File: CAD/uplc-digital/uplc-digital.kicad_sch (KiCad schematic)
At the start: 34 parts, among them J1 Conn_01x06_Pin, J2 SM12B-GHS-TB(LF)(SN), U1 AP63201WU, U2 TBD62003AFWG, U3 ESP32-C3-WROOM-02, Y1 32.768khz 3215 12.5pf

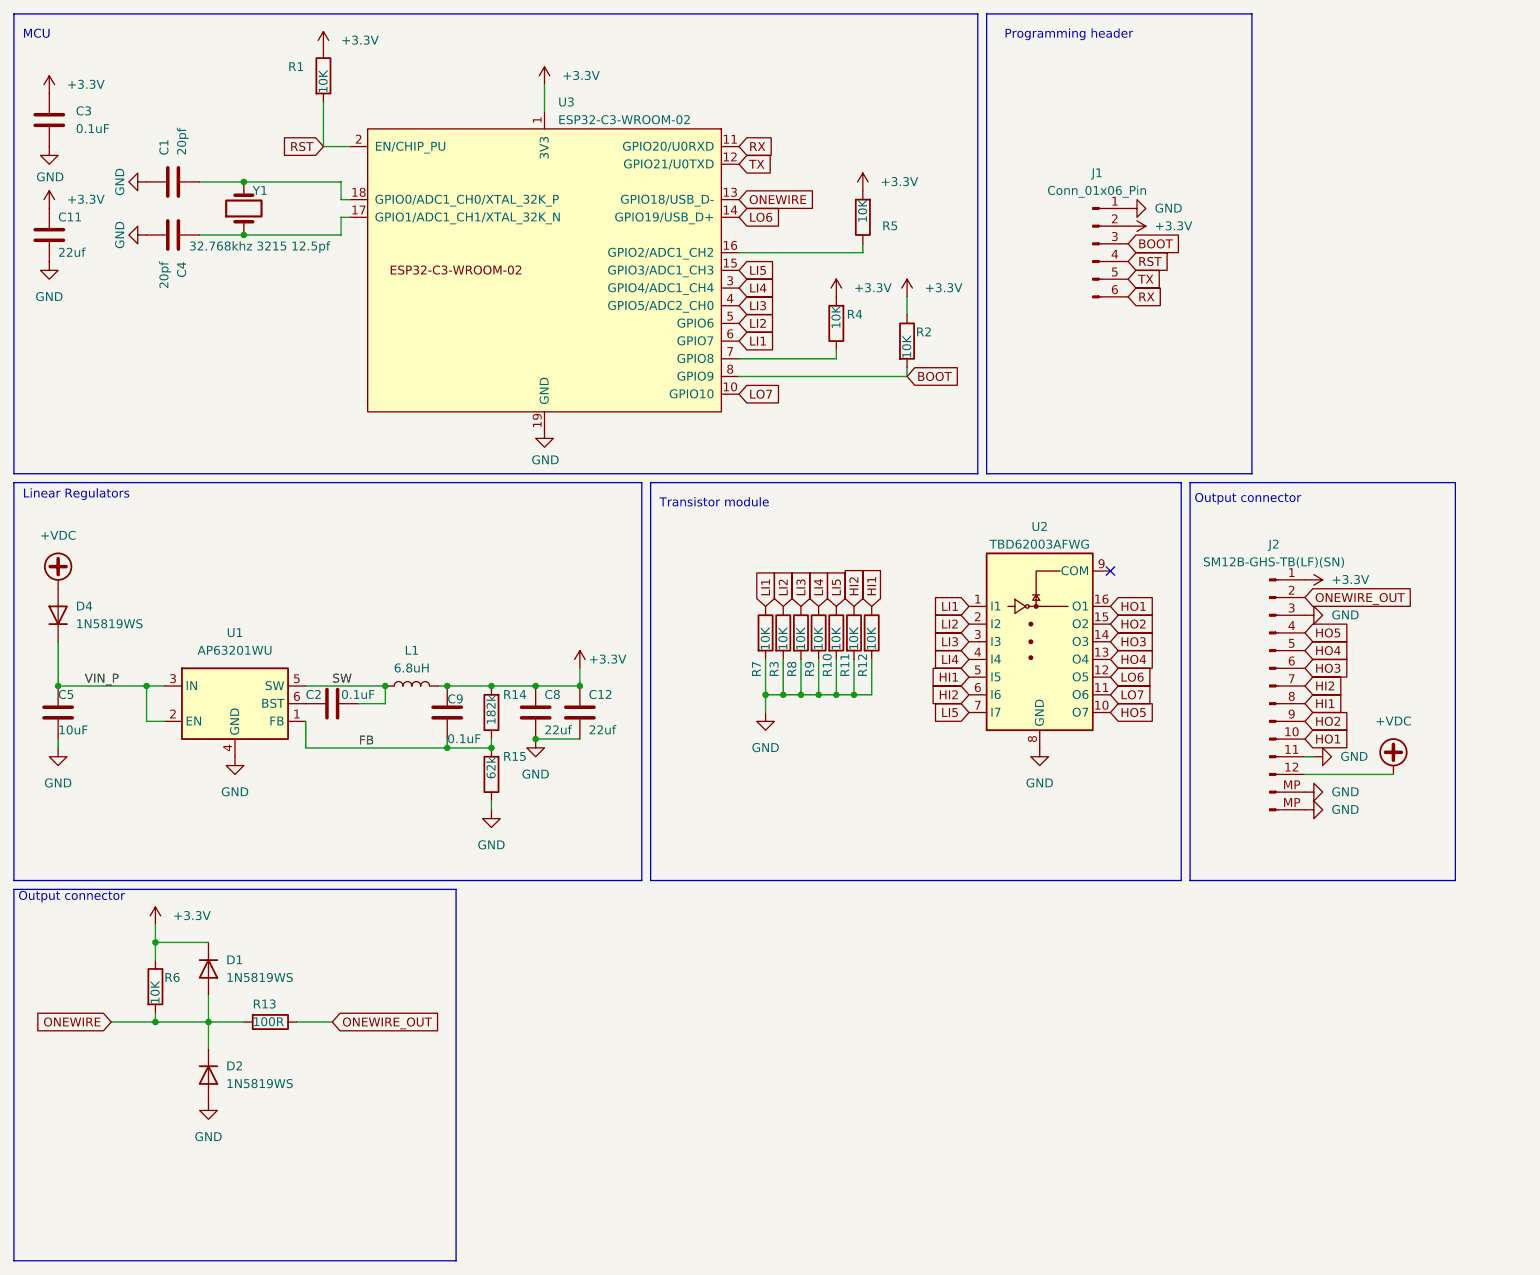
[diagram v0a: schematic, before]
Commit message: WIP rev 1.1
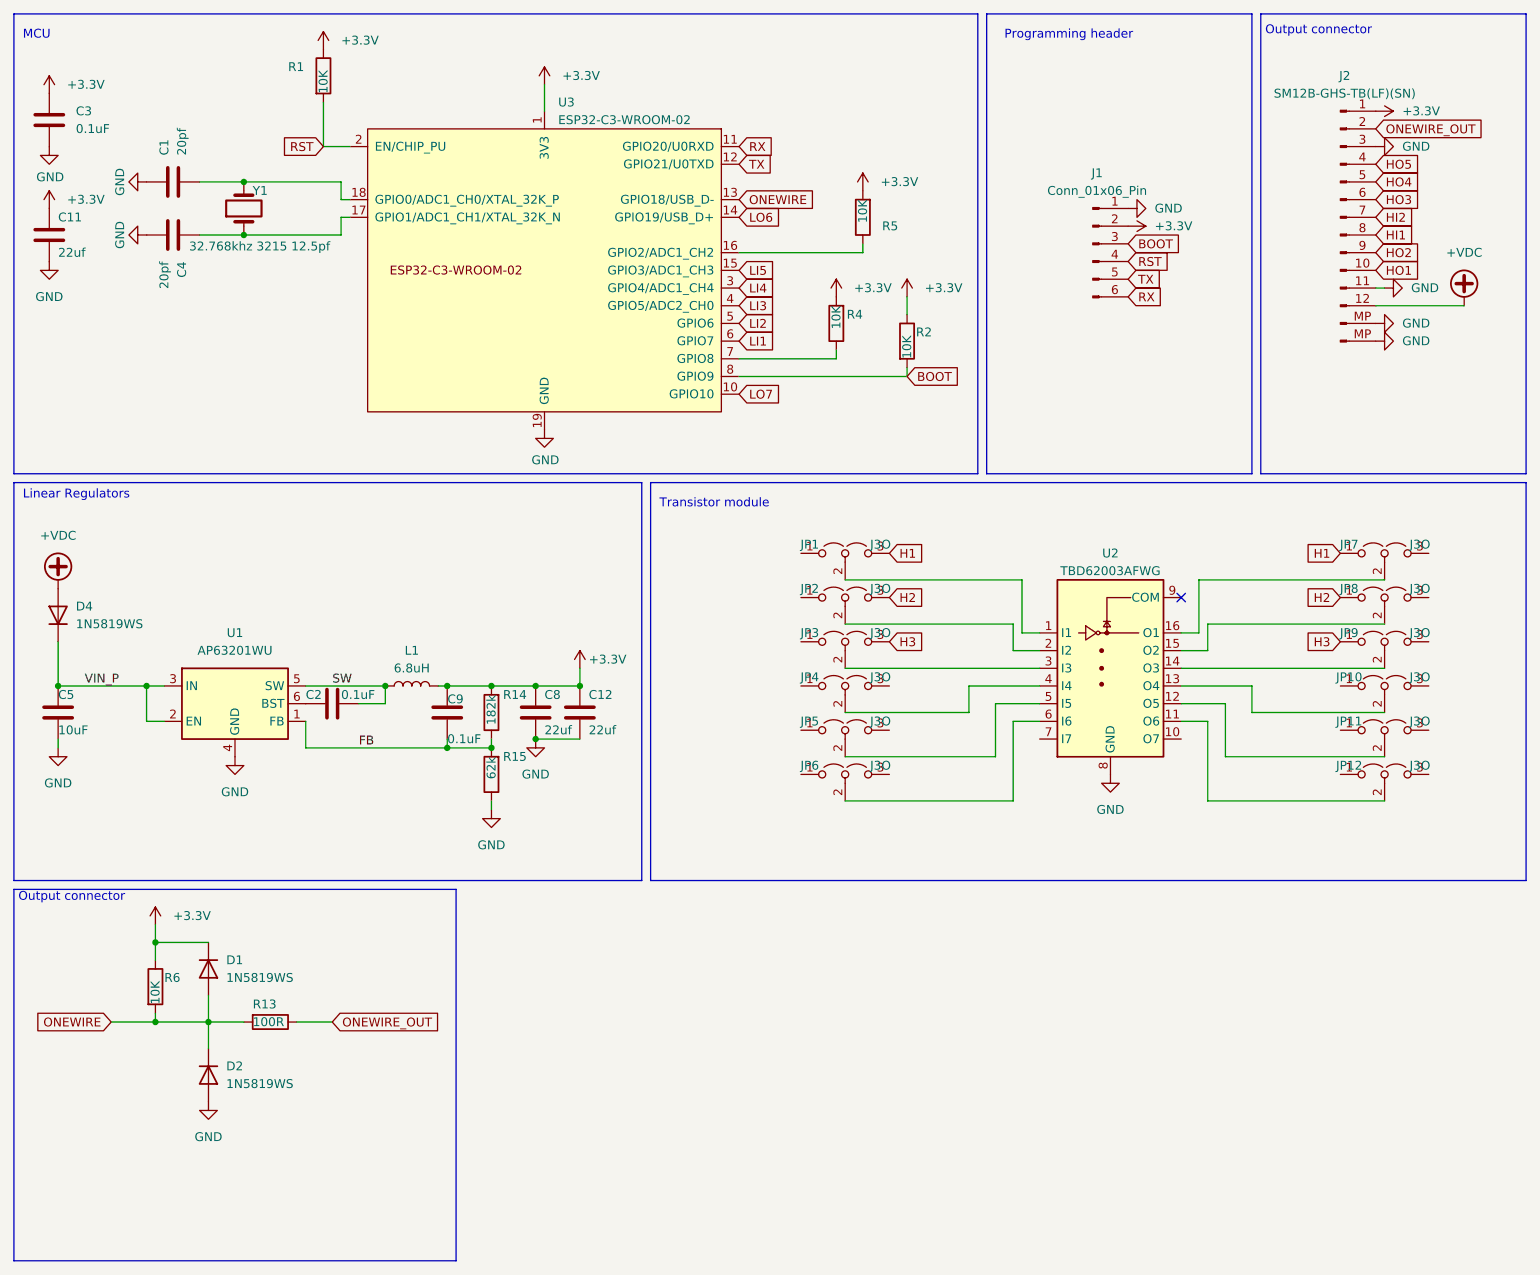
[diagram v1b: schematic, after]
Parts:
- removed R10, R11, R12, R3, R7, R8, R9: 10K, Resistor_SMD:R_0402_1005Metric, symbol Library:R
- added JP1, JP10, JP11, JP12, JP2, JP3, JP4, JP5, JP6, JP7, JP8, JP9: J3O, Jumper:SolderJumper-3_P1.3mm_Open_Pad1.0x1.5mm_NumberLabels, symbol Jumper:Jumper_3_Open
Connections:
- net HI1: no longer U2.5 (I5)
- net HI2: no longer U2.6 (I6)
- net HO1: no longer U2.16 (O1)
- net HO2: no longer U2.15 (O2)
- net HO3: no longer U2.14 (O3)
- net HO4: no longer U2.13 (O4)
- net HO5: no longer U2.10 (O7)
- net LI1: no longer U2.1 (I1)
- net LI2: no longer U2.2 (I2)
- net LI3: no longer U2.3 (I3)
- net LI4: no longer U2.4 (I4)
- net LI5: no longer U2.7 (I7)
- net LO6: no longer U2.12 (O5)
- net LO7: no longer U2.11 (O6)
- new net: JP10.2 (C), U2.13 (O4)
- new net: JP6.2 (C), U2.6 (I6)
- new net: JP3.2 (C), U2.3 (I3)
- new net: JP1.2 (C), U2.1 (I1)
- new net: JP7.2 (C), U2.16 (O1)
- new net: JP11.2 (C), U2.12 (O5)
- new net: JP4.2 (C), U2.4 (I4)
- new net: JP5.2 (C), U2.5 (I5)
- new net: JP8.2 (C), U2.15 (O2)
- new net: JP2.2 (C), U2.2 (I2)
- new net: JP9.2 (C), U2.14 (O3)
- new net: JP12.2 (C), U2.11 (O6)
- new net H1: JP1.3 (B), JP7.1 (A)
- new net H2: JP2.3 (B), JP8.1 (A)
- new net H3: JP3.3 (B), JP9.1 (A)
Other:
- moved on the sheet: J2, U2

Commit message: Rev 1.1 Schem PCB done
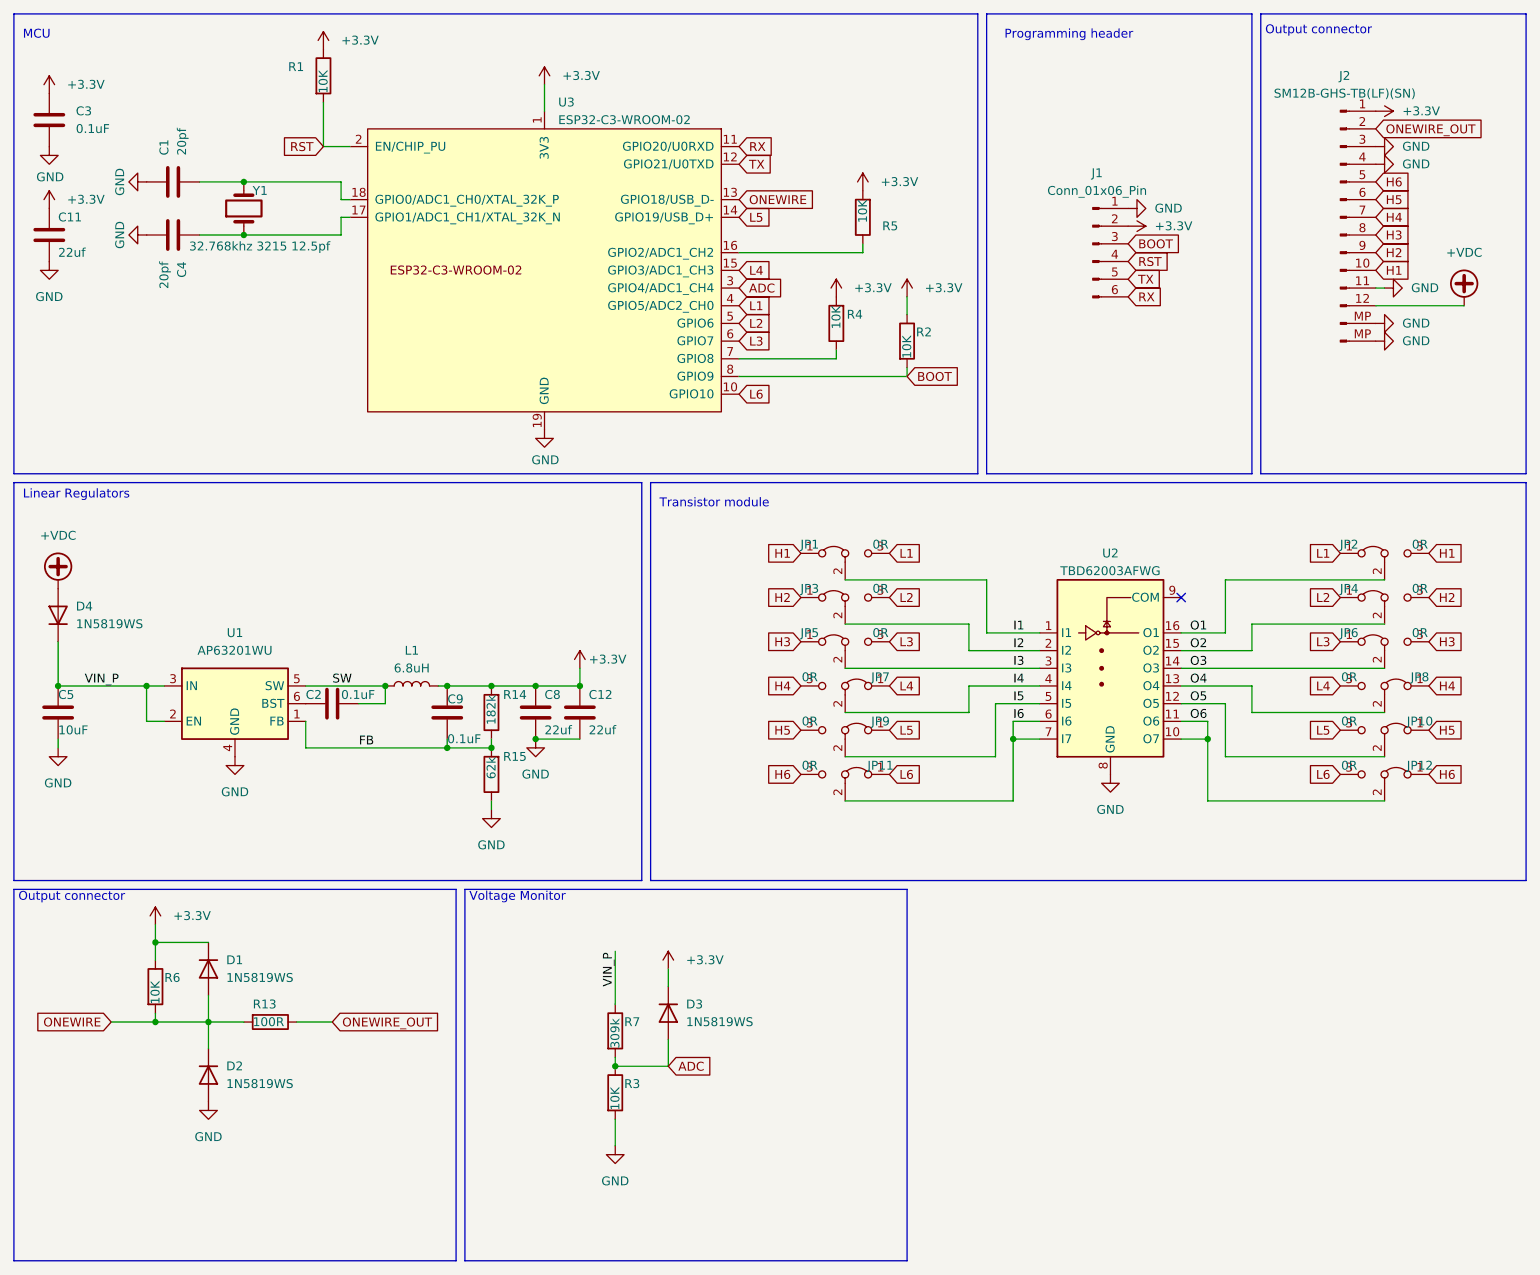
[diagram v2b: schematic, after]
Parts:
- removed JP1, JP10, JP11, JP12, JP2, JP3, JP4, JP5, JP6, JP7, JP8, JP9: J3O, Jumper:SolderJumper-3_P1.3mm_Open_Pad1.0x1.5mm_NumberLabels, symbol Jumper:Jumper_3_Open
- added D3: 1N5819WS, Diode_SMD:D_SOD-323, symbol Library:1N4148WS
- added JP1, JP10, JP11, JP12, JP2, JP3, JP4, JP5, JP6, JP7, JP8, JP9: 0R, Jumper:SolderJumper-3_P1.3mm_BridgedSMD12_0402, symbol Jumper:Jumper_3_Bridged12
- added R3: 10K, Resistor_SMD:R_0402_1005Metric, symbol Library:R
- added R7: 309k, Resistor_SMD:R_0402_1005Metric, symbol Library:R
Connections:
- net HI1 is gone; now on net H3: J2.8 (Pin_8)
- net HO1 is gone; now on net H1: J2.10 (Pin_10)
- net HO2 is gone; now on net H2: J2.9 (Pin_9)
- net HO5 is gone; now on net GND: J2.4 (Pin_4)
- net +3.3V: now also D3.1 (K)
- net GND: now also R3.2
- net H1: now also JP1.1 (A), JP2.3 (B)
- net H2: now also JP3.1 (A), JP4.3 (B)
- net H3: now also JP5.1 (A), JP6.3 (B)
- net VIN_P: now also R7.1
- net O4: now reaches U2.13 (O4)
- net O4: now also JP8.2 (C)
- net I6: now reaches U2.6 (I6)
- net I6: now also U2.7 (I7), JP11.2 (C)
- net I3: now reaches U2.3 (I3)
- net I3: now also JP5.2 (C)
- net I1: now reaches U2.1 (I1)
- net I1: now also JP1.2 (C)
- net O1: now reaches U2.16 (O1)
- net O1: now also JP2.2 (C)
- net O5: now reaches U2.12 (O5)
- net O5: now also JP10.2 (C)
- net I4: now reaches U2.4 (I4)
- net I4: now also JP7.2 (C)
- net I5: now reaches U2.5 (I5)
- net I5: now also JP9.2 (C)
- net O2: now reaches U2.15 (O2)
- net O2: now also JP4.2 (C)
- net I2: now reaches U2.2 (I2)
- net I2: now also JP3.2 (C)
- net O3: now reaches U2.14 (O3)
- net O3: now also JP6.2 (C)
- net O6: now reaches U2.11 (O6)
- net O6: now also U2.10 (O7), JP12.2 (C)
- net HI2 renamed H4
- net H4: now also JP7.3 (B), JP8.1 (A)
- net HO3 renamed H5
- net H5: now also JP10.1 (A), JP9.3 (B)
- net HO4 renamed H6
- net H6: now also JP11.3 (B), JP12.1 (A)
- net LI1 renamed L3
- net L3: now also JP5.3 (B), JP6.1 (A)
- net LI2 renamed L2
- net L2: now also JP3.3 (B), JP4.1 (A)
- net LI3 renamed L1
- net L1: now also JP1.3 (B), JP2.1 (A)
- net LI4 renamed ADC
- net ADC: now also D3.2 (A), R3.1, R7.2
- net LI5 renamed L4
- net L4: now also JP7.1 (A), JP8.3 (B)
- net LO6 renamed L5
- net L5: now also JP10.3 (B), JP9.1 (A)
- net LO7 renamed L6
- net L6: now also JP11.1 (A), JP12.3 (B)
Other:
- note added: "Voltage Monitor"

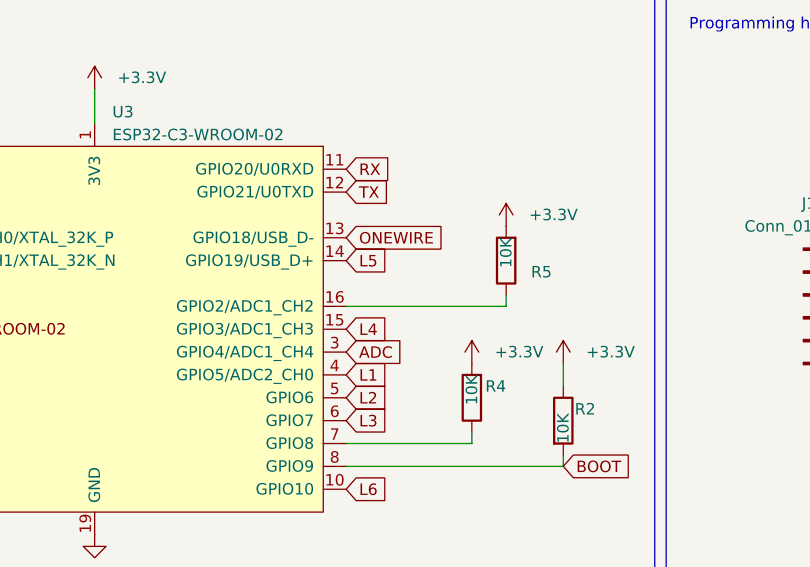
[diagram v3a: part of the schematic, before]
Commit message: Rev 1.2
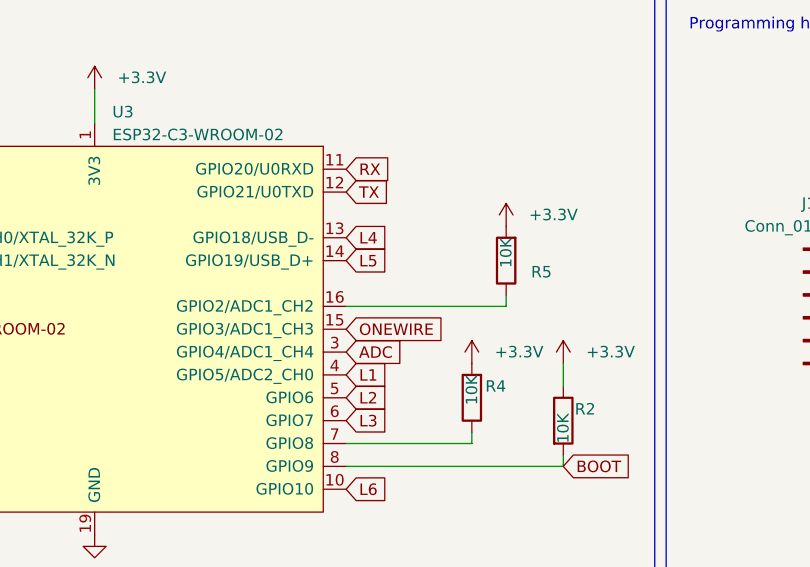
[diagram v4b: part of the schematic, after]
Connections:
- net L4: now also U3.13 (GPIO18/USB_D-); no longer U3.15 (GPIO3/ADC1_CH3)
- net ONEWIRE: now also U3.15 (GPIO3/ADC1_CH3); no longer U3.13 (GPIO18/USB_D-)
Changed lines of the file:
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@@
     (title "uPLC-Digital")
     (date "2024-02-22")
-    (rev "1.0.0")
+    (rev "1.2.0")
     (company "Drawn by FNB")
     (comment 1 "Thanks to https://github.com/PricelessToolkit/ESPClicker for inspiration")
@@
     )
   )
-  (global_label "ONEWIRE" (shape input) (at 120.65 43.18 0) (fields_autoplaced)
+  (global_label "ONEWIRE" (shape input) (at 120.65 53.34 0) (fields_autoplaced)
     (effects (font (size 1.27 1.27)) (justify left))
-    (property "Intersheetrefs" "${INTERSHEET_REFS}" (at 131.9204 43.18 0)
+    (property "Intersheetrefs" "${INTERSHEET_REFS}" (at 131.9204 53.34 0)
       (effects (font (size 1.27 1.27)) (justify left) hide)
     )
@@
     )
   )
-  (global_label "L4" (shape input) (at 120.65 53.34 0) (fields_autoplaced)
+  (global_label "L4" (shape input) (at 120.65 43.18 0) (fields_autoplaced)
     (effects (font (size 1.27 1.27)) (justify left))
-    (property "Intersheetrefs" "${INTERSHEET_REFS}" (at 125.8728 53.34 0)
+    (property "Intersheetrefs" "${INTERSHEET_REFS}" (at 125.8728 43.18 0)
       (effects (font (size 1.27 1.27)) (justify left) hide)
     )

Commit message: Panelization changes
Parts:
- JP1, JP10, JP11, JP12, JP2, JP3, JP4, JP5, JP6, JP7, JP8, JP9: LCSC Part # (none) -> C102746
- R7: LCSC Part # (none) -> C159040

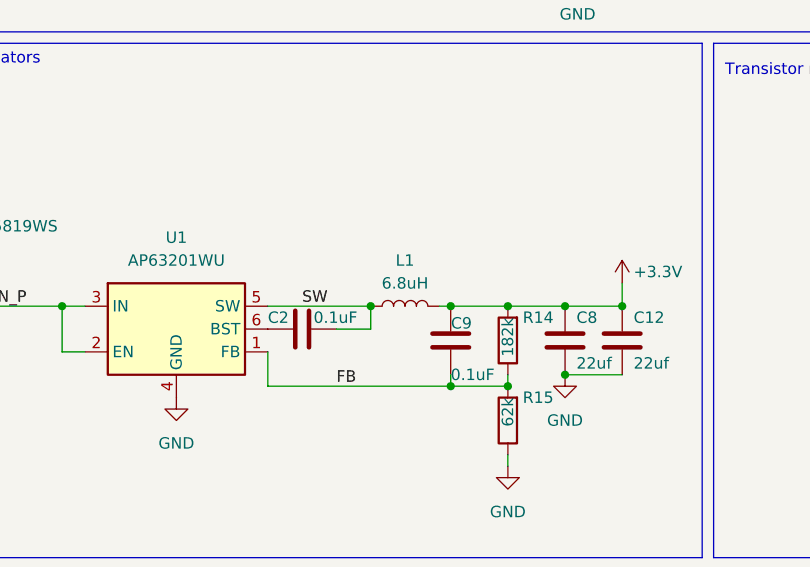
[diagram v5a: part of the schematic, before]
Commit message: Feat: V1.1
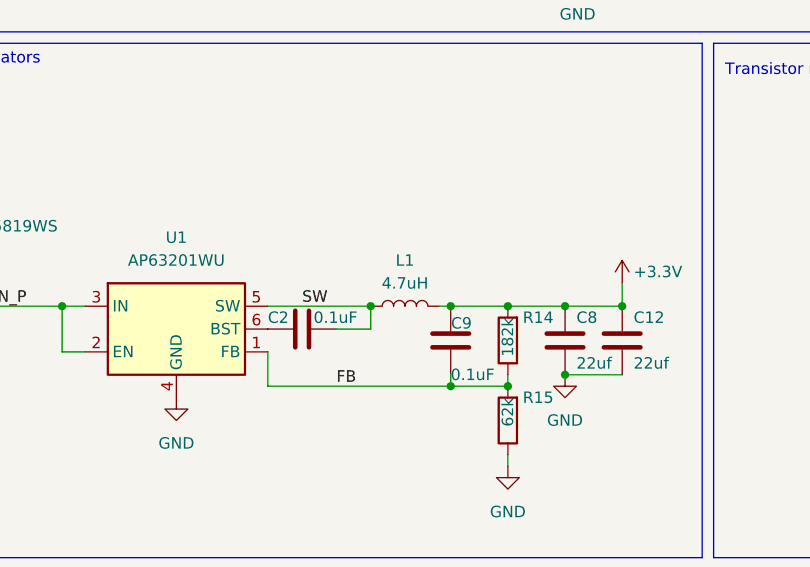
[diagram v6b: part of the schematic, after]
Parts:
- C1, C4: Generic (none) -> x; MPN (none) -> 0402CG200J500NT
- C11, C12, C8: Generic (none) -> x; MPN (none) -> GRM155R60J226ME11D
- C2, C3, C9: Generic (none) -> x; LCSC Part # C307331 -> C77020; MPN (none) -> GRM155R71H104KE14D
- C5: Generic (none) -> x; MPN (none) -> GRM21BR6YA106KE43L
- D1, D2, D3, D4: MPN (none) -> 1N5819WS
- J2: MPN (none) -> SM12B-GHS-TB(LF)(SN)
- JP1, JP10, JP11, JP12, JP2, JP3, JP4, JP5, JP6, JP7, JP8, JP9: Generic (none) -> x; MPN (none) -> RTT02000JTH
- L1: value 6.8uH -> 4.7uH; Generic (none) -> x; LCSC Part # C98340 -> C82314; MPN (none) -> LQM2HPN4R7MG0L
- R1, R2, R3, R4, R5, R6: Generic (none) -> x; MPN (none) -> 0402WGF1002TCE
- R13: Generic (none) -> x; MPN (none) -> 0402WGF1000TCE
- R14: Generic (none) -> x; MPN (none) -> 0402WGF1823TCE
- R15: Generic (none) -> x; MPN (none) -> RC0402FR-0762KL
- R7: Generic (none) -> x; MPN (none) -> RTT023093FTH
- U1: MPN (none) -> AP63201WU-7
- U2: MPN (none) -> TBD62003AFWG
- U3: MPN (none) -> ESP32-C3-WROOM-02-N4
- Y1: MPN (none) -> Q13FC13500004
